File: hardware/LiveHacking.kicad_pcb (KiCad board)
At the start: 2 copper layers, 83.5 x 83.5 mm, 4 parts

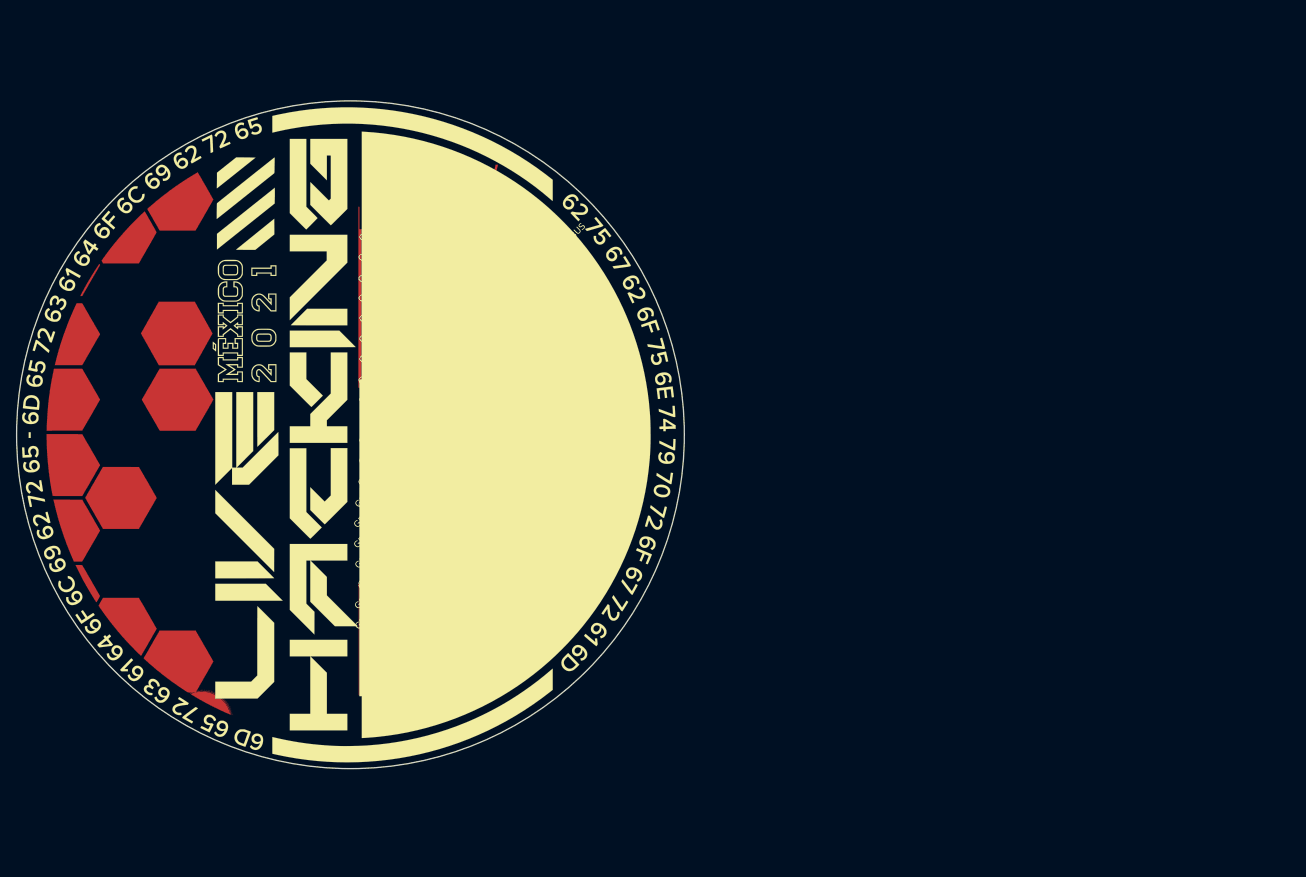
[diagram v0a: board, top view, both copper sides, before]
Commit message: update project schmeatic start routing
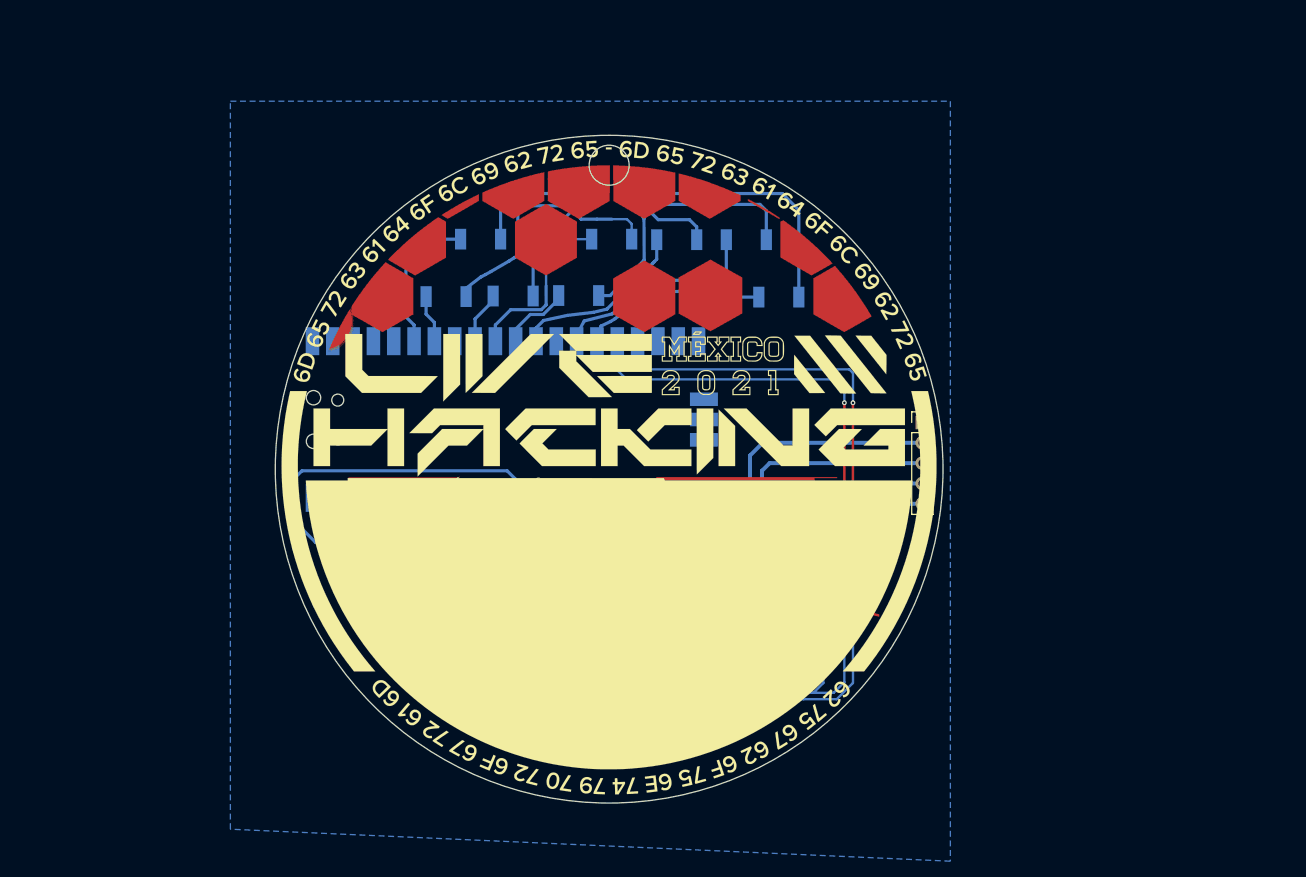
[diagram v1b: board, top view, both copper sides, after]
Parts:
- removed REF**: RPi_Pico_SMD_TH, MCU_RaspberryPi_and_Boards:RPi_Pico_SMD_TH
- added BT1: Battery_Cell, Badge-LiveHacking:12BH423GR, B.Cu at (141.4, 122.1)
- added D1: MBR120, Diode_SMD:D_SOD-123F, B.Cu at (87.0, 108.1)
- added D2: LED, Badge-LiveHacking:LYT77K-K2M1-NoHole, B.Cu at (101.3, 67.2)
- added D3: LED, Badge-LiveHacking:LYT77K-K2M1-NoHole, B.Cu at (97.0, 74.4)
- added D4: LED, Badge-LiveHacking:LYT77K-K2M1-NoHole, B.Cu at (117.7, 67.2)
- added D5: LED, Badge-LiveHacking:LYT77K-K2M1-NoHole, B.Cu at (105.3, 74.4)
- added D6: LED, Badge-LiveHacking:LYT77K-K2M1-NoHole, B.Cu at (138.6, 74.5)
- added D7: LED, Badge-LiveHacking:LYT77K-K2M1-NoHole, B.Cu at (113.5, 74.3)
- added D8: LED, Badge-LiveHacking:LYT77K-K2M1-NoHole, B.Cu at (134.5, 67.3)
- added D9: LED, Badge-LiveHacking:LYT77K-K2M1-NoHole, B.Cu at (125.8, 67.3)
- added J1: Conn_01x05, Connector_PinHeader_2.54mm:PinHeader_1x05_P2.54mm_Vertical, F.Cu at (156.5, 90.2)
- added RN1: R_Pack04, Resistor_SMD:R_Array_Convex_4x0603, B.Cu at (112.2, 60.6)
- added RN2: R_Pack04, Resistor_SMD:R_Array_Convex_4x0603, B.Cu at (122.0, 60.6)
- added SW1: RST, Button_Switch_SMD:SW_SPST_TL3342, B.Cu at (81.3, 108.8)
- added SW2: SW_Push, Button_Switch_SMD:SW_SPST_TL3342, F.Cu at (132.0, 126.0)
- added SW3: SW_Push, Button_Switch_SMD:SW_SPST_TL3342, F.Cu at (102.7, 126.0)
- added U1: Pico, Badge-LiveHacking:RPi_Pico_SMD_TH, B.Cu at (104.4, 89.8)
- moved G*** 84.3 mm to (124.5, 133.3)
- moved G*** 79.5 mm to (108.4, 131.8)
- moved Ref** 33.0 mm to (117.3, 95.6), turned to 270 degrees
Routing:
- net /BTN2: track 0.00 -> 121.3 mm, vias 0 -> 4
- net /BTN1: track 0.00 -> 117.8 mm, vias 0 -> 3
- net +3V3: track 0.00 -> 78.9 mm
- net /ADC0: track 0.00 -> 65.8 mm
- net +BATT: track 0.00 -> 53.9 mm
- net /GPIO19: track 0.00 -> 51.0 mm
- net /GPIO18: track 0.00 -> 48.9 mm
- net /RUN_RESET: track 0.00 -> 46.6 mm
- net Net-(D6-Pad1): track 0.00 -> 29.6 mm
- net /LED7: track 0.00 -> 27.9 mm
- net /LED8: track 0.00 -> 24.2 mm
- net /LED6: track 0.00 -> 23.8 mm
- net /LED4: track 0.00 -> 23.7 mm
- net Net-(D3-Pad1): track 0.00 -> 21.7 mm
- net /LED1: track 0.00 -> 20.2 mm
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- added copper zone on B.Cu, net GND
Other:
- outline, holes or cut-outs redrawn

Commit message: update holder
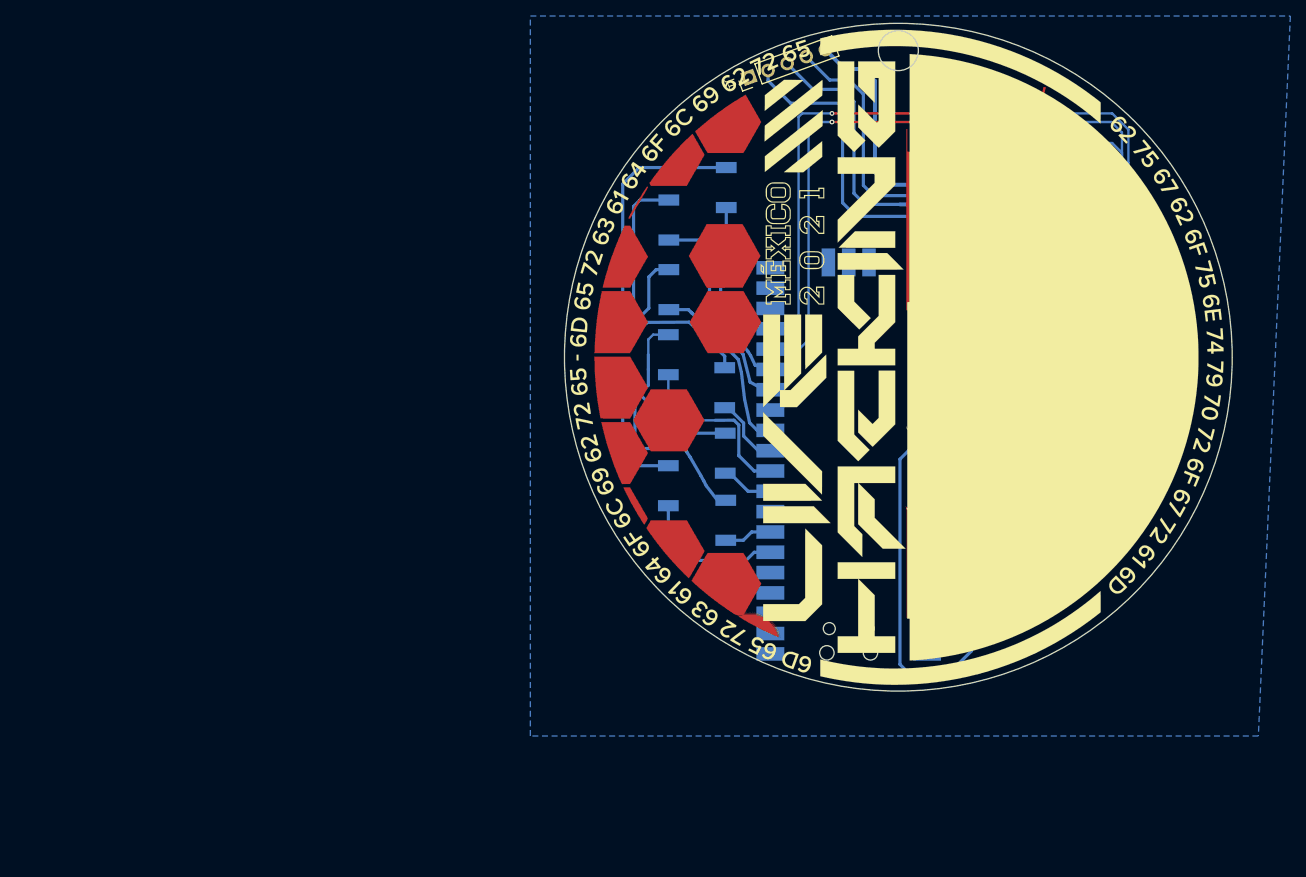
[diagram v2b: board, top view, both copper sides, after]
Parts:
- moved G*** 90.7 mm to (189.3, 91.0), turned to 270 degrees
- moved G*** 88.4 mm to (190.8, 74.9), turned to 270 degrees
- moved SW3 86.0 mm to (183.5, 96.7), turned to 90 degrees
- moved SW1 85.5 mm to (166.2, 118.0), turned to 200 degrees
- moved D1 78.7 mm to (165.6, 112.3), turned to 20 degrees
- moved SW2 78.1 mm to (183.5, 67.3), turned to 90 degrees
- moved BT1 74.7 mm to (179.6, 58.0), turned to 90 degrees
- moved J1 48.3 mm to (134.8, 47.0), turned to 110 degrees
- moved D3 44.8 mm to (131.9, 102.4), turned to 270 degrees
- moved U1 43.2 mm to (147.3, 95.0), turned to 0 degrees
- moved D2 38.7 mm to (124.7, 98.1), turned to 270 degrees
- moved Ref** 38.2 mm to (153.1, 82.0), turned to 0 degrees
- moved D5 33.0 mm to (131.9, 94.0), turned to 270 degrees
- moved RN1 27.2 mm to (118.1, 87.2), turned to 0 degrees
- moved D7 21.6 mm to (131.8, 85.8), turned to 270 degrees
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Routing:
- net +3V3: track 78.9 -> 90.1 mm
- net /ADC0: track 65.8 -> 74.7 mm
- net /GPIO18: track 48.9 -> 56.6 mm
- net /GPIO19: track 51.0 -> 58.7 mm
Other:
- outline, holes or cut-outs redrawn
